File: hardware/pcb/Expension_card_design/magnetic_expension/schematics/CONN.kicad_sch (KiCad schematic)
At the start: 8 parts, among them J1 550910374

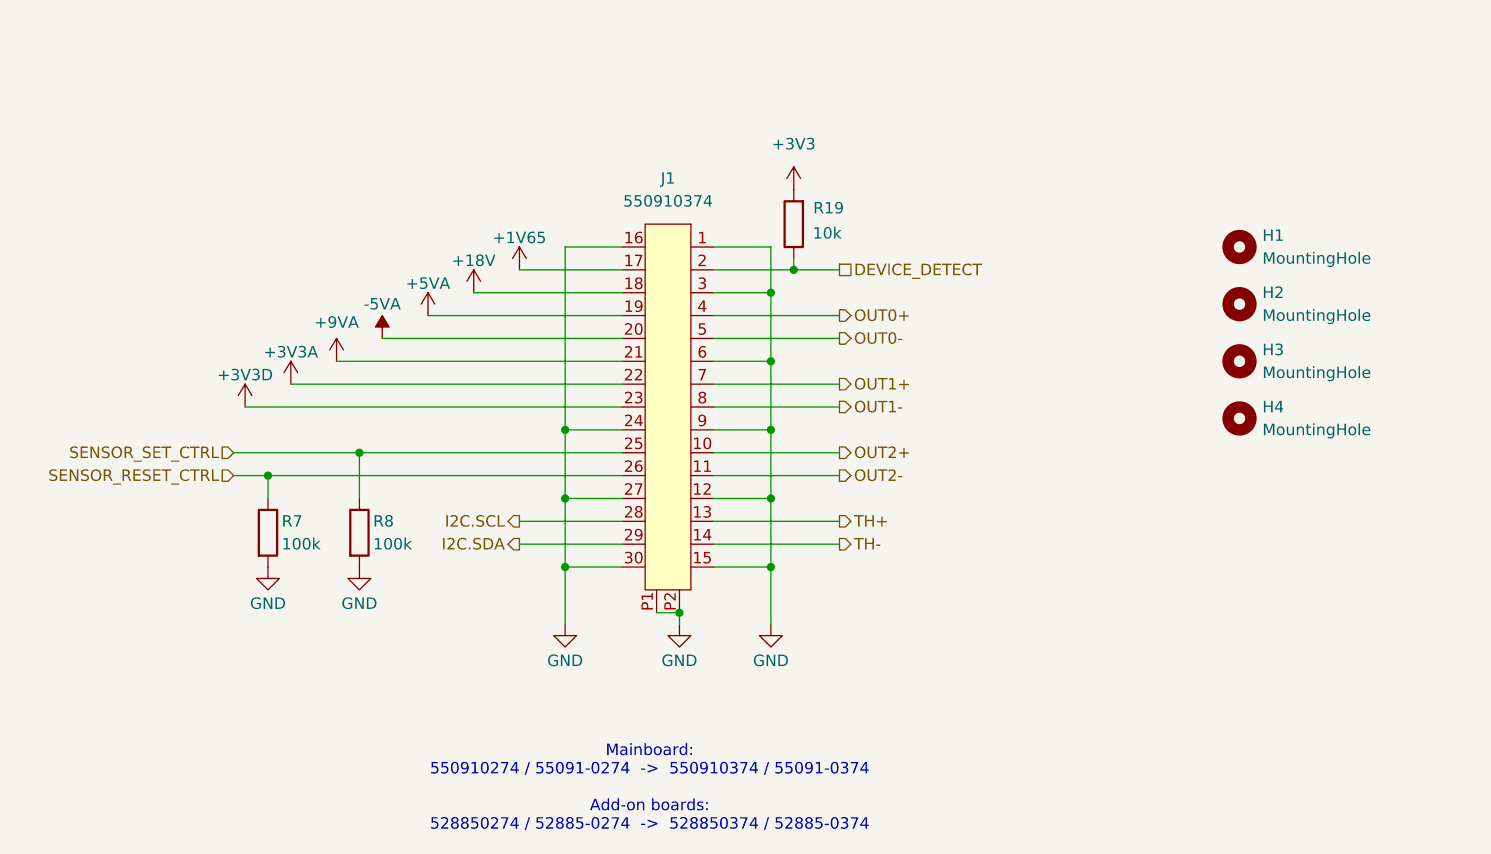
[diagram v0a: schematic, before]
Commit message: Work in progress rev2
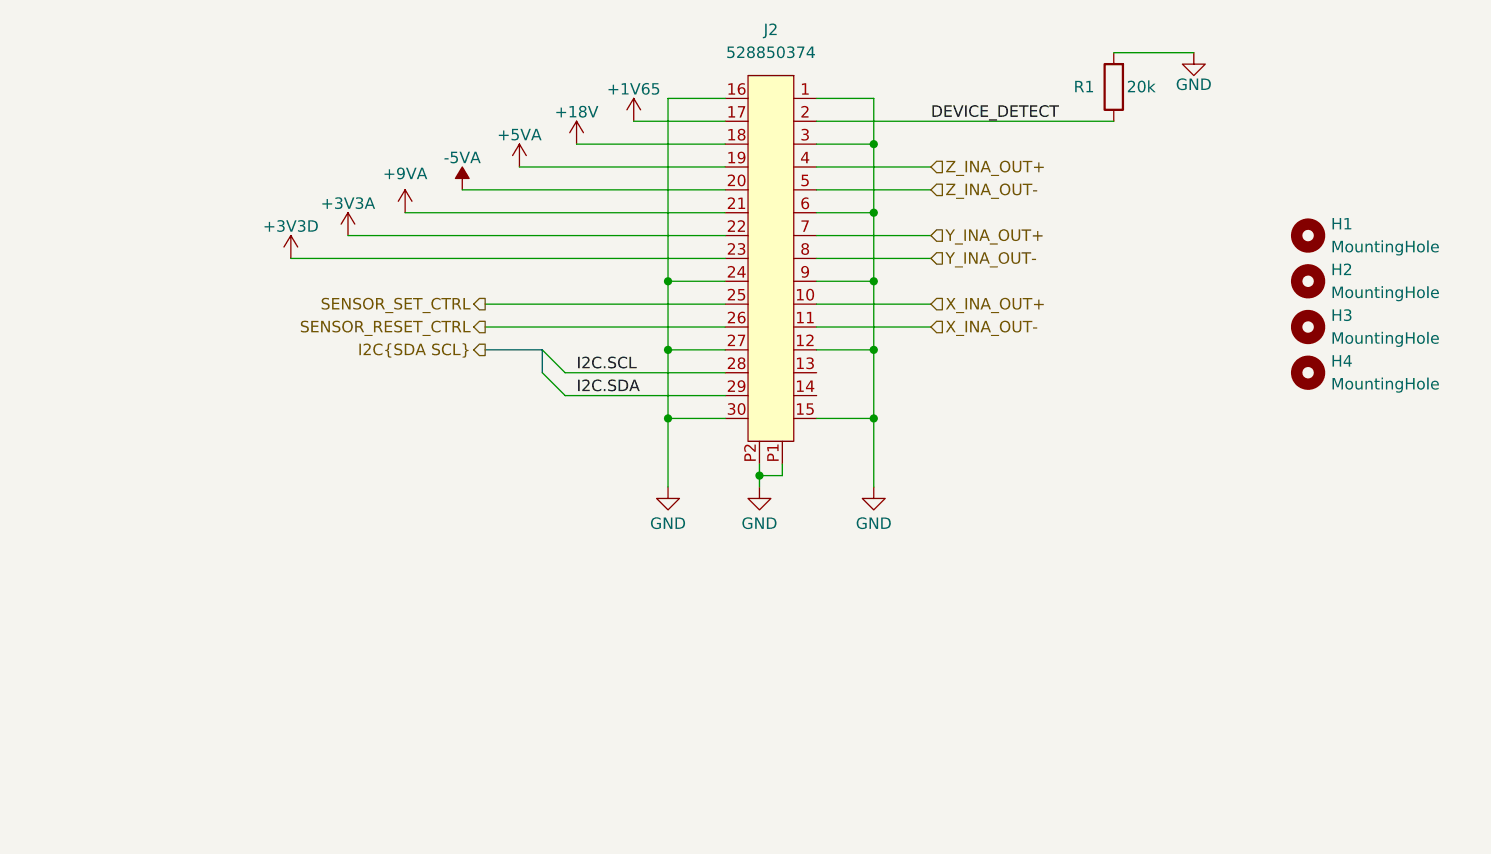
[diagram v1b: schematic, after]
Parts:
- removed J1: 550910374, magnode_footprints:CONN_MOLEX_02x15_55091-0374, symbol magnode_symbols:55091-0374
- removed R19: 10k, Resistor_SMD:R_0603_1608Metric, symbol Device:R
- removed R7, R8: 100k, Resistor_SMD:R_0603_1608Metric, symbol Device:R
- added J2: 528850374, magnode_footprints:CONN_MOLEX_02x15_52885-0374, symbol magnode_symbols:52885-0374
- added R1: 20k, Resistor_SMD:R_0603_1608Metric, symbol Device:R
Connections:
- net +18V: now also J2.18
- net +1V65: now also J2.17
- net +3V3A: now also J2.22
- net +3V3D: now also J2.23
- net +5VA: now also J2.19
- net +9VA: now also J2.21
- net -5VA: now also J2.20
- net DEVICE_DETECT: now also J2.2, R1.1
- net GND: now also J2.1, J2.12, J2.15, J2.16, J2.24, J2.27, J2.3, J2.30, J2.6, J2.9, J2.P1, J2.P2, R1.2
- net I2C.SCL: now also J2.28
- net I2C.SDA: now also J2.29
- net SENSOR_RESET_CTRL: now also J2.26
- net SENSOR_SET_CTRL: now also J2.25
- new net X_INA_OUT+: J2.10
- new net X_INA_OUT-: J2.11
- new net Y_INA_OUT+: J2.7
- new net Y_INA_OUT-: J2.8
- new net Z_INA_OUT+: J2.4
- new net Z_INA_OUT-: J2.5
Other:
- note removed: "Mainboard: 550910274 / 55091-0274 -> 550910374 / 55091-0374 Add-on boards: 528850274 / 52885-0274 -> 528850374 / 52885-0374"
